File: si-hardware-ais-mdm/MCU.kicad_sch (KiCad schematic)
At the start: 21 parts, among them J4 USB_C_Receptacle_USB2.0_16P, SW1 SW_Push, SW2 SW_Push, U6 ESP32-C6-MINI-1-H4, U7 LIS331HH

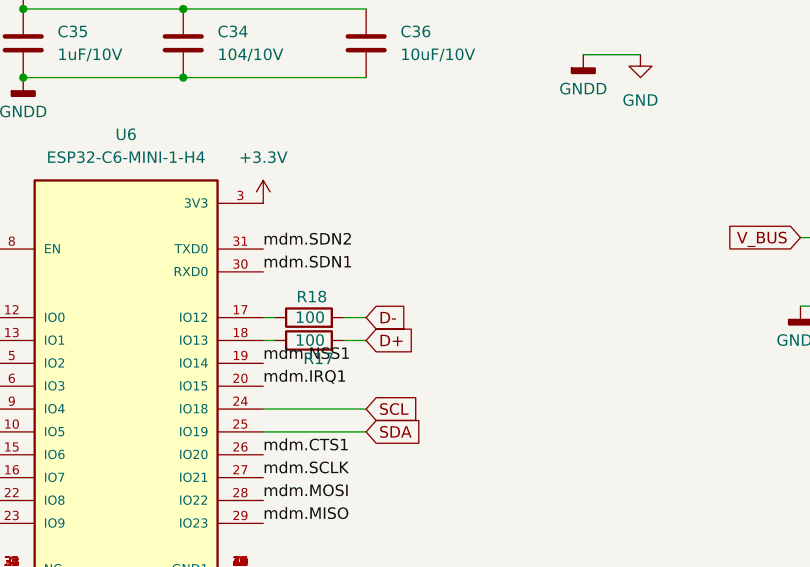
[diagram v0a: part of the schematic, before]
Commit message: routing 3
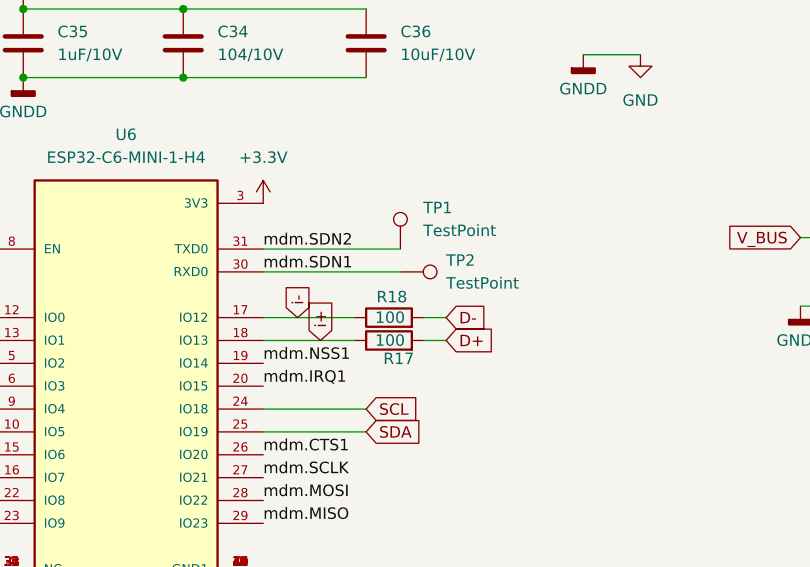
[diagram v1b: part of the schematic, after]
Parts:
- added TP1, TP2: TestPoint, TestPoint:TestPoint_Pad_D1.0mm, symbol Connector:TestPoint
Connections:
- net mdm.SDN1: now also TP2.1
- net mdm.SDN2: now also TP1.1
- net i+: now reaches R17.1, U6.18 (IO13)
- net i-: now reaches R18.1, U6.17 (IO12)
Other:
- moved on the sheet: R17, R18
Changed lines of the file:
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@@
 		)
 	)
-	(wire
-		(pts
-			(xy 125.73 91.44) (xy 138.43 91.44)
-		)
-		(stroke
-			(width 0)
-			(type default)
-		)
-	)
 	(bus
 		(pts
@@
 	(wire
 		(pts
-			(xy 125.73 93.98) (xy 138.43 93.98)
-		)
-		(stroke
-			(width 0)
-			(type default)
-		)
-	)
-	(wire
-		(pts
 			(xy 95.25 57.15) (xy 95.25 60.96)
 		)
@@
 	(wire
 		(pts
-			(xy 125.73 88.9) (xy 138.43 88.9)
+			(xy 125.73 139.7) (xy 140.97 139.7)
 		)
 		(stroke
@@
 	(wire
 		(pts
-			(xy 125.73 139.7) (xy 140.97 139.7)
+			(xy 125.73 88.9) (xy 138.43 88.9)
 		)
 		(stroke
@@
 		)
 	)
+	(wire
+		(pts
+			(xy 125.73 93.98) (xy 138.43 93.98)
+		)
+		(stroke
+			(width 0)
+			(type default)
+		)
+	)
 	(bus
 		(pts
@@
 	(wire
 		(pts
-			(xy 168.91 76.2) (xy 170.18 76.2)
+			(xy 168.91 76.2) (xy 179.07 76.2)
+		)
+		(stroke
+			(width 0)
+			(type default)
+		)
+	)
+	(wire
+		(pts
+			(xy 125.73 91.44) (xy 138.43 91.44)
 		)
 		(stroke
@@
 	(wire
 		(pts
+			(xy 168.91 71.12) (xy 184.15 71.12)
+		)
+		(stroke
+			(width 0)
+			(type default)
+		)
+	)
+	(wire
+		(pts
 			(xy 228.6 67.31) (xy 232.41 67.31)
 		)
@@
 	(wire
 		(pts
+			(xy 125.73 86.36) (xy 138.43 86.36)
+		)
+		(stroke
+			(width 0)
+			(type default)
+		)
+	)
+	(wire
+		(pts
 			(xy 72.39 125.73) (xy 88.9 125.73)
 		)
@@
 	(wire
 		(pts
-			(xy 125.73 86.36) (xy 138.43 86.36)
+			(xy 125.73 96.52) (xy 138.43 96.52)
 		)
 		(stroke
@@
 	(wire
 		(pts
-			(xy 125.73 96.52) (xy 138.43 96.52)
+			(xy 168.91 68.58) (xy 184.15 68.58)
 		)
 		(stroke
@@
 	(wire
 		(pts
-			(xy 168.91 78.74) (xy 170.18 78.74)
+			(xy 168.91 78.74) (xy 179.07 78.74)
 		)
 		(stroke
@@
 	(wire
 		(pts
-			(xy 177.8 78.74) (xy 180.34 78.74)
+			(xy 186.69 78.74) (xy 189.23 78.74)
 		)
 		(stroke
@@
 	(wire
 		(pts
-			(xy 177.8 76.2) (xy 180.34 76.2)
+			(xy 186.69 76.2) (xy 189.23 76.2)
 		)
 		(stroke
@@
 	(global_label "D-"
 		(shape input)
-		(at 180.34 76.2 0)
+		(at 189.23 76.2 0)
 		(fields_autoplaced yes)
 		(effects
@@
 		)
 		(property "Intersheetrefs" "${INTERSHEET_REFS}"
-			(at 186.1676 76.2 0)
+			(at 195.0576 76.2 0)
 			(effects
 				(font
@@
 		)
 	)
+	(global_label "i-"
+		(shape input)
+		(at 172.72 76.2 90)
+		(fields_autoplaced yes)
+		(effects
+			(font
+				(size 1.27 1.27)
+			)
+			(justify left)
+		)
+		(property "Intersheetrefs" "${INTERSHEET_REFS}"
+			(at 172.72 71.0376 90)
+			(effects
+				(font
+					(size 1.27 1.27)
+				)
+				(justify left)
+				(hide yes)
+			)
+		)
+	)
 	(global_label "SCL"
 		(shape input)
@@
 		)
 	)
+	(global_label "i+"
+		(shape input)
+		(at 175.26 78.74 90)
+		(fields_autoplaced yes)
+		(effects
+			(font
+				(size 1.27 1.27)
+			)
+			(justify left)
+		)
+		(property "Intersheetrefs" "${INTERSHEET_REFS}"
+			(at 175.26 73.5776 90)
+			(effects
+				(font
+					(size 1.27 1.27)
+				)
+				(justify left)
+				(hide yes)
+			)
+		)
+	)
 	(global_label "D+"
 		(shape input)
@@
 	(global_label "D+"
 		(shape input)
-		(at 180.34 78.74 0)
+		(at 189.23 78.74 0)
 		(fields_autoplaced yes)
 		(effects
@@
 		)
 		(property "Intersheetrefs" "${INTERSHEET_REFS}"
-			(at 186.1676 78.74 0)
+			(at 195.0576 78.74 0)
 			(effects
 				(font
@@
 	)
 	(symbol
+		(lib_id "Connector:TestPoint")
+		(at 184.15 68.58 0)
+		(unit 1)
+		(exclude_from_sim no)
+		(in_bom yes)
+		(on_board yes)
+		(dnp no)
+		(fields_autoplaced yes)
+		(property "Reference" "TP1"
+			(at 186.69 64.0079 0)
+			(effects
+				(font
+					(size 1.27 1.27)
+				)
+				(justify left)
+			)
+		)
+		(property "Value" "TestPoint"
+			(at 186.69 66.5479 0)
+			(effects
+				(font
+					(size 1.27 1.27)
+				)
+				(justify left)
+			)
+		)
+		(property "Footprint" "TestPoint:TestPoint_Pad_D1.0mm"
+			(at 189.23 68.58 0)
+			(effects
+				(font
+					(size 1.27 1.27)
+				)
+				(hide yes)
+			)
+		)
+		(property "Datasheet" "~"
+			(at 189.23 68.58 0)
+			(effects
+				(font
+					(size 1.27 1.27)
+				)
+				(hide yes)
+			)
+		)
+		(property "Description" "test point"
+			(at 184.15 68.58 0)
+			(effects
+				(font
+					(size 1.27 1.27)
+				)
+				(hide yes)
+			)
+		)
+		(pin "1"
+		)
+		(instances
+			(project ""
+				(path "/97f80214-d5cc-4a35-9cac-bb1ff8330c6a/487f8325-78ac-466b-85b4-df92bc0f13d9"
+					(reference "TP1")
+					(unit 1)
+				)
+			)
+		)
+	)
+	(symbol
 		(lib_id "power:+3.3V")
 		(at 35.56 130.81 0)
@@
 	(symbol
 		(lib_id "Device:R")
-		(at 173.99 78.74 90)
+		(at 182.88 78.74 90)
 		(unit 1)
 		(exclude_from_sim no)
@@
 		(dnp no)
 		(property "Reference" "R17"
-			(at 176.784 80.772 90)
+			(at 185.674 80.772 90)
 			(effects
 				(font
@@
 		)
 		(property "Value" "100"
-			(at 175.768 78.74 90)
+			(at 184.658 78.74 90)
 			(effects
 				(font
@@
 		)
 		(property "Footprint" "Resistor_SMD:R_0402_1005Metric"
-			(at 173.99 80.518 90)
+			(at 182.88 80.518 90)
 			(effects
 				(font
@@
 		)
 		(property "Datasheet" "~"
-			(at 173.99 78.74 0)
+			(at 182.88 78.74 0)
 			(effects
 				(font
@@
 		)
 		(property "Description" "Resistor"
-			(at 173.99 78.74 0)
+			(at 182.88 78.74 0)
 			(effects
 				(font
@@
 	)
 	(symbol
+		(lib_id "Connector:TestPoint")
+		(at 184.15 71.12 270)
+		(unit 1)
+		(exclude_from_sim no)
+		(in_bom yes)
+		(on_board yes)
+		(dnp no)
+		(fields_autoplaced yes)
+		(property "Reference" "TP2"
+			(at 189.23 69.8499 90)
+			(effects
+				(font
+					(size 1.27 1.27)
+				)
+				(justify left)
+			)
+		)
+		(property "Value" "TestPoint"
+			(at 189.23 72.3899 90)
+			(effects
+				(font
+					(size 1.27 1.27)
+				)
+				(justify left)
+			)
+		)
+		(property "Footprint" "TestPoint:TestPoint_Pad_D1.0mm"
+			(at 184.15 76.2 0)
+			(effects
+				(font
+					(size 1.27 1.27)
+				)
+				(hide yes)
+			)
+		)
+		(property "Datasheet" "~"
+			(at 184.15 76.2 0)
+			(effects
+				(font
+					(size 1.27 1.27)
+				)
+				(hide yes)
+			)
+		)
+		(property "Description" "test point"
+			(at 184.15 71.12 0)
+			(effects
+				(font
+					(size 1.27 1.27)
+				)
+				(hide yes)
+			)
+		)
+		(pin "1"
+		)
+		(instances
+			(project "si-hardware-ais-mdm"
+				(path "/97f80214-d5cc-4a35-9cac-bb1ff8330c6a/487f8325-78ac-466b-85b4-df92bc0f13d9"
+					(reference "TP2")
+					(unit 1)
+				)
+			)
+		)
+	)
+	(symbol
 		(lib_id "power:+3.3V")
 		(at 95.25 49.53 0)
@@
 	(symbol
 		(lib_id "Device:R")
-		(at 173.99 76.2 90)
+		(at 182.88 76.2 90)
 		(unit 1)
 		(exclude_from_sim no)
@@
 		(dnp no)
 		(property "Reference" "R18"
-			(at 176.022 73.914 90)
+			(at 184.912 73.914 90)
 			(effects
 				(font
@@
 		)
 		(property "Value" "100"
-			(at 175.768 76.2 90)
+			(at 184.658 76.2 90)
 			(effects
 				(font
@@
 		)
 		(property "Footprint" "Resistor_SMD:R_0402_1005Metric"
-			(at 173.99 77.978 90)
+			(at 182.88 77.978 90)
 			(effects
 				(font
@@
 		)
 		(property "Datasheet" "~"
-			(at 173.99 76.2 0)
+			(at 182.88 76.2 0)
 			(effects
 				(font
@@
 		)
 		(property "Description" "Resistor"
-			(at 173.99 76.2 0)
+			(at 182.88 76.2 0)
 			(effects
 				(font
